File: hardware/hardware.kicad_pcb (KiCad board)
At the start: 2 copper layers, 32 x 42 mm, 17 parts, among them J1 OUTPUT, U1 MP2303ADN

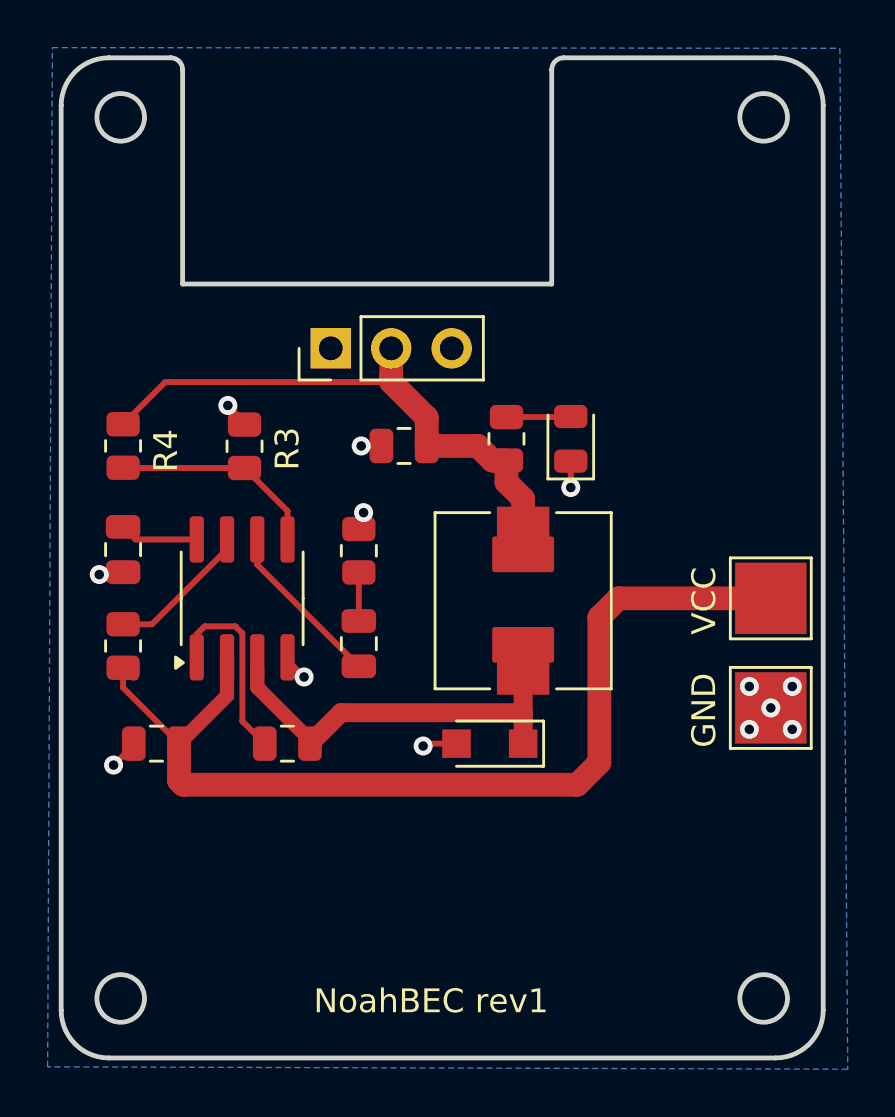
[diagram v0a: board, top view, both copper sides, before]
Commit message: update rev2
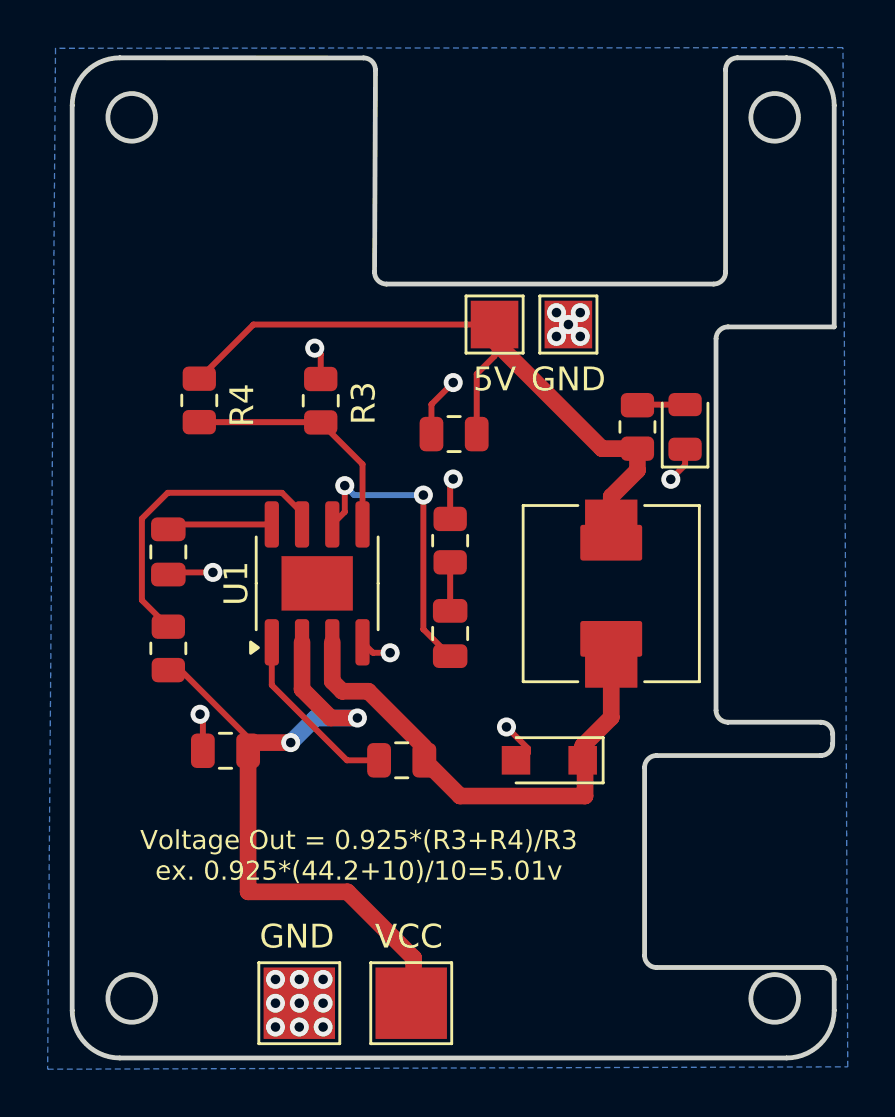
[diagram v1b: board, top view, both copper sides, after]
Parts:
- removed J1: OUTPUT, Connector_PinHeader_2.54mm:PinHeader_1x03_P2.54mm_Vertical
- added 5V: 5V OUTPUT, TestPoint:TestPoint_Pad_2.0x2.0mm, F.Cu at (143.9, 74.9)
- added GND: GND OUTPUT, TestPoint:TestPoint_Pad_2.0x2.0mm, F.Cu at (147.0, 74.9)
- U1: footprint Package_SO:SOIC-8_3.9x4.9mm_P1.27mm -> Package_SO:SOIC-8-1EP_3.9x4.9mm_P1.27mm_EP2.29x3mm
- moved GND 23.4 mm to (135.7, 103.4)
- moved VCC 22.7 mm to (140.4, 103.4)
- moved R5 5.52 mm to (149.9, 79.2)
- moved C4 4.85 mm to (140.0, 93.2)
- moved D2 4.83 mm to (151.9, 79.2)
- moved R1 3.86 mm to (142.0, 84.0)
- moved C2 3.86 mm to (142.0, 87.9)
- moved R3 3.73 mm to (136.6, 78.1)
- moved R4 3.73 mm to (131.5, 78.1)
- moved L1 3.71 mm to (148.8, 86.2)
- moved U1 3.21 mm to (136.4, 85.8)
- moved C6 2.92 mm to (132.6, 92.8)
- moved D1 2.60 mm to (146.2, 93.2)
- moved C5 2.16 mm to (142.2, 79.5)
- moved C1 1.90 mm to (130.2, 84.5)
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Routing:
- net Net-(J5-Pin_1): track 43.0 -> 31.2 mm, vias 0 -> 2
- net Net-(U1-EN): track 6.08 -> 13.0 mm
- net 5V: track 23.3 -> 30.2 mm
- net Net-(U1-COMP): track 7.09 -> 12.5 mm, vias 0 -> 2
- net GND: track 8.67 -> 13.9 mm, vias 13 -> 22
- net Net-(D1-K): track 16.2 -> 20.6 mm
- net Net-(U1-BS): track 8.94 -> 7.61 mm
- net Net-(U1-FB): track 8.85 -> 10.1 mm
- net Net-(U1-SS): track 3.31 -> 4.43 mm
- net Net-(D2-A): track 2.71 -> 2.19 mm
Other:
- outline, holes or cut-outs redrawn
- board text added: "NoahBEC rev2"
- board text added: "Voltage Out = 0.925*(R3+R4)/R3 ex. 0.925*(44.2+10)/10=5.01v"
- board text removed: "NoahBEC rev1"
- board text removed: "Voltage Out = 0.925 * ( R3 + R4 ) / R3 ex. 0.925 * ( 44.2 + 10 ) / 10 = 5.01v"
